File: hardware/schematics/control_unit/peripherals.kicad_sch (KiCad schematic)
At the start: 4 parts, among them U11 MAX487E

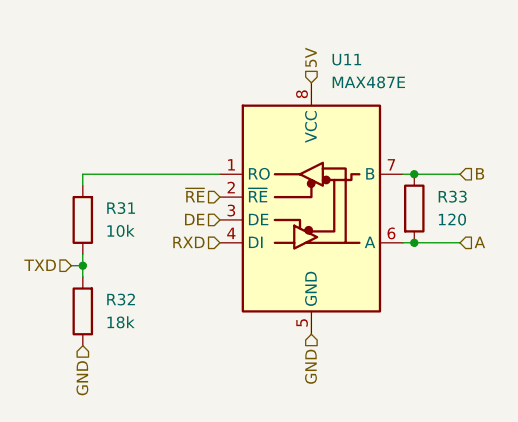
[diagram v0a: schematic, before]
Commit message: !refactor
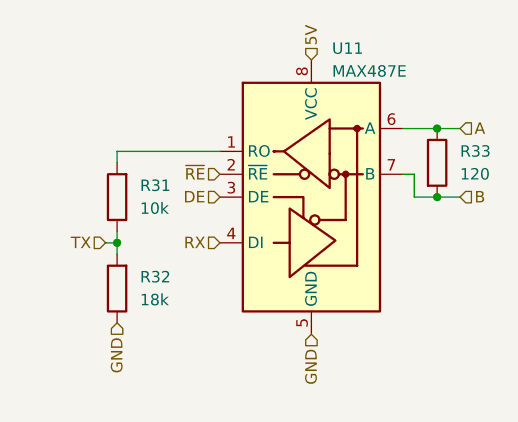
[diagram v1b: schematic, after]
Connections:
- net A: now also R33.1; no longer R33.2
- net B: now also R33.2; no longer R33.1
- net RXD renamed RX
- net TXD renamed TX
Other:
- moved on the sheet: R31, R32, R33
